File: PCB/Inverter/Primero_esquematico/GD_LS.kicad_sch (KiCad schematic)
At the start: 46 parts, among them T7 750317595, U40 LM25180QNGURQ1, U41 UCC21750QDWRQ1, U42 LP2951-5.0_VSSOP

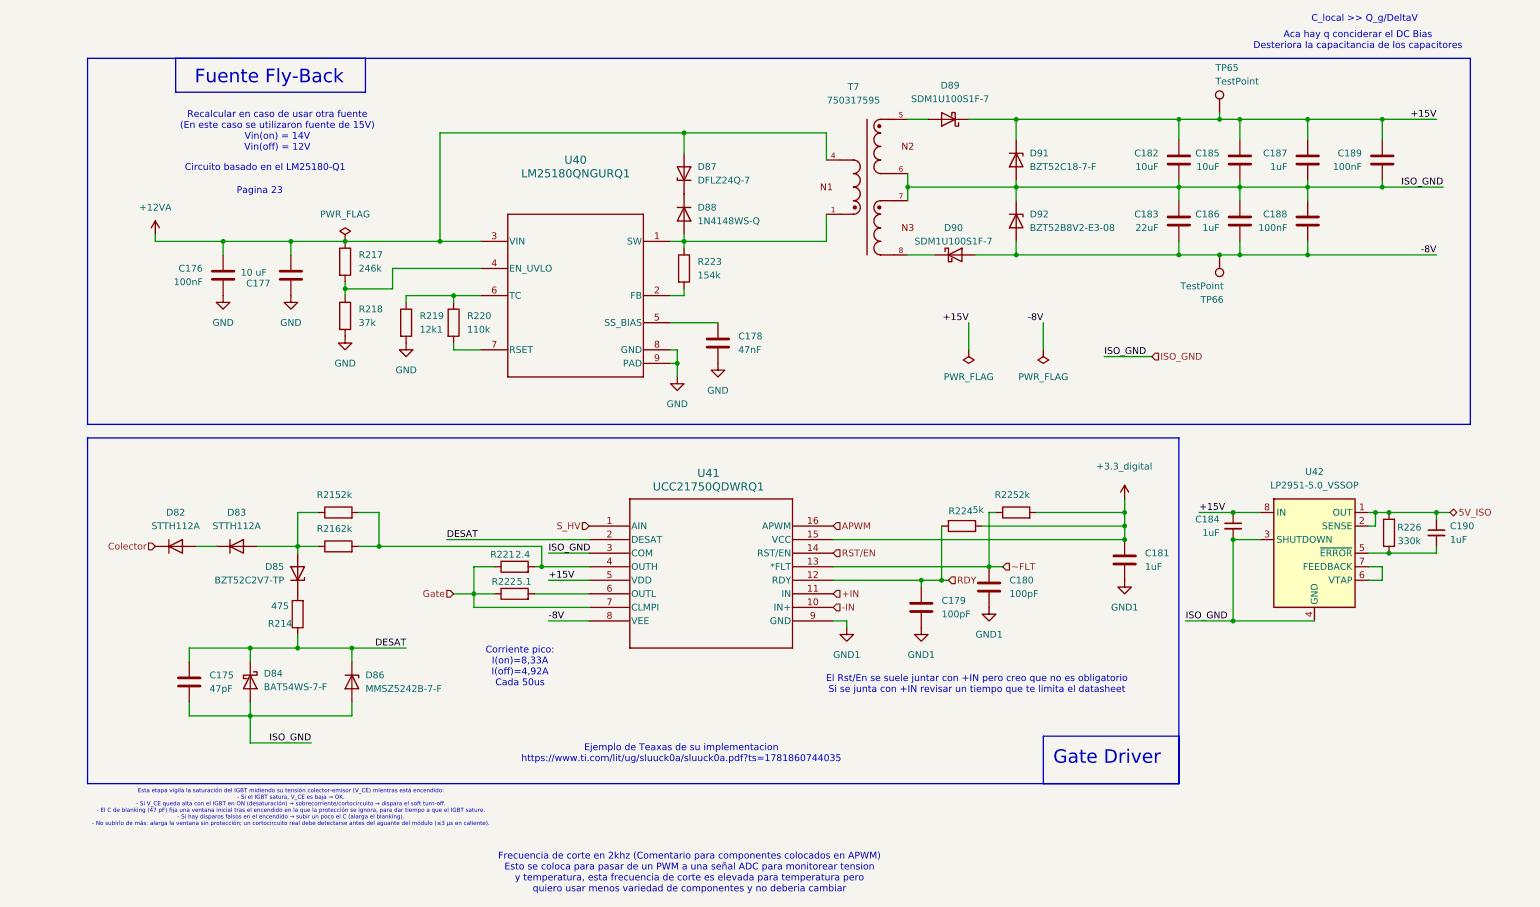
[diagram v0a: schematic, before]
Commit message: Corregi cosas de la placa
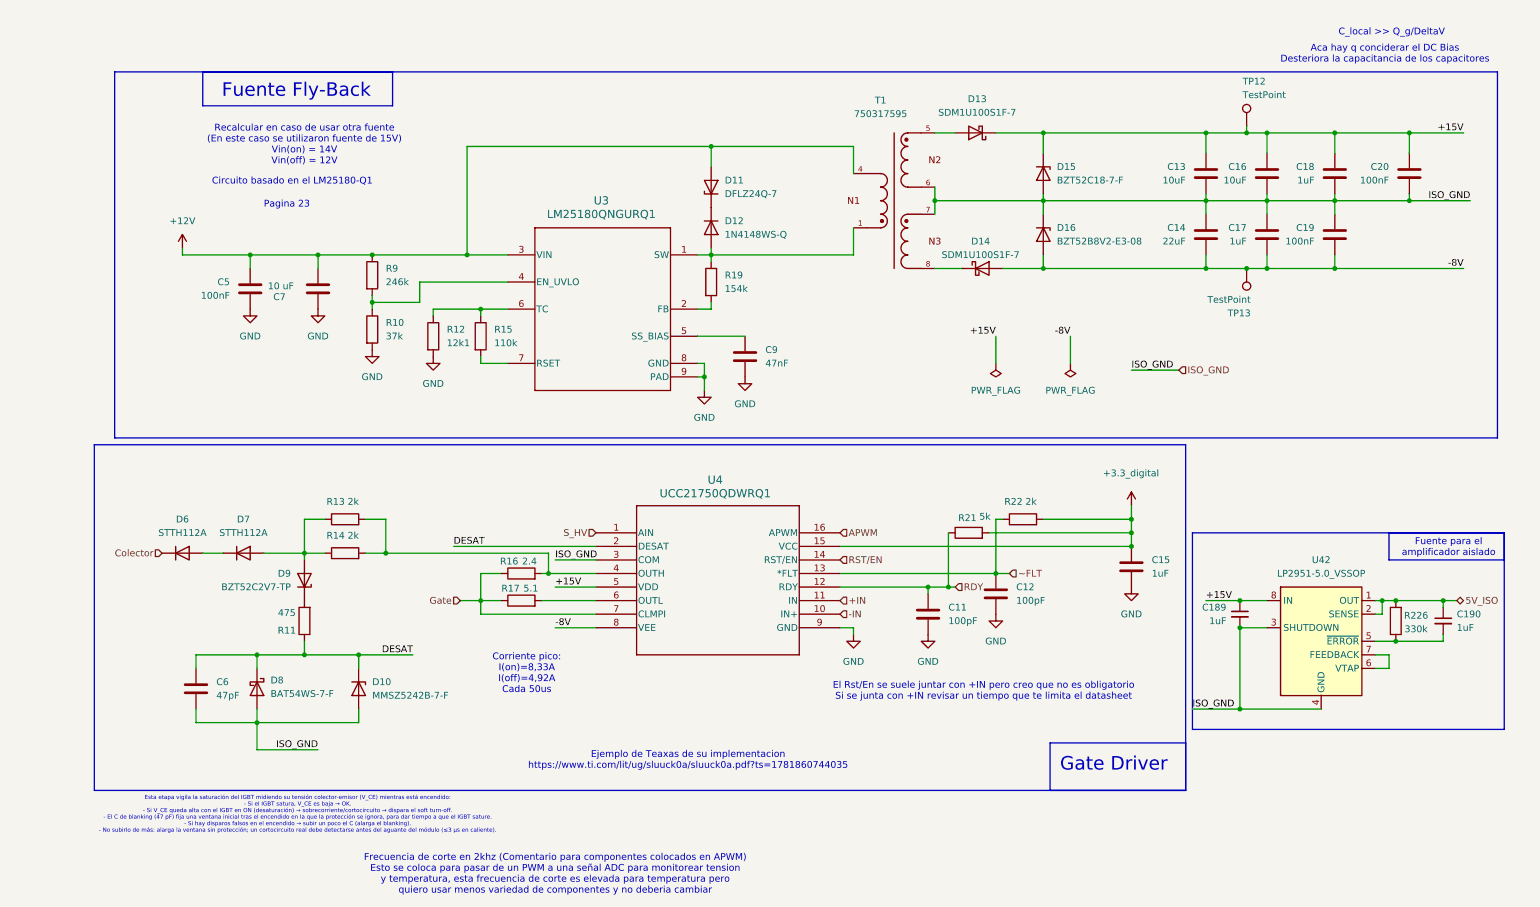
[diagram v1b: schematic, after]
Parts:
- removed C175: 47pF, Capacitor_SMD:C_0603_1608Metric_Pad1.08x0.95mm_HandSolder, symbol Device:C
- removed C176, C188, C189: 100nF, Capacitor_SMD:C_0402_1005Metric, symbol Device:C
- removed C177: 10 uF, Capacitor_SMD:C_1206_3216Metric, symbol Device:C
- removed C178: 47nF, Capacitor_SMD:C_0402_1005Metric_Pad0.74x0.62mm_HandSolder, symbol Device:C
- removed C179, C180: 100pF, Capacitor_SMD:C_0402_1005Metric, symbol Device:C
- removed C181: 1uF, Capacitor_SMD:C_0603_1608Metric, symbol Device:C
- removed C182, C185: 10uF, Capacitor_SMD:C_1210_3225Metric, symbol Device:C
- removed C183: 22uF, Capacitor_SMD:C_1210_3225Metric, symbol Device:C
- removed C184: 1uF, Capacitor_SMD:C_0603_1608Metric, symbol Device:C_Small
- removed C186, C187: 1uF, Capacitor_SMD:C_0805_2012Metric, symbol Device:C
- removed D82, D83: STTH112A, Diode_SMD:D_SOD-323F, symbol Device:D
- removed D84: BAT54WS-7-F, Diode_SMD:D_SOD-323_HandSoldering, symbol Device:D_Schottky
- removed D85: BZT52C2V7-TP, Diode_SMD:D_SOD-123, symbol Device:D_Zener
- removed D86: MMSZ5242B-7-F, Diode_SMD:D_SOD-123, symbol Device:D_Zener
- removed D87: DFLZ24Q-7, Diode_SMD:D_PowerDI-123, symbol Device:D_Zener
- removed D88: 1N4148WS-Q, Diode_SMD:D_SOD-323F, symbol Device:D
- removed D89, D90: SDM1U100S1F-7, Diode_SMD:D_SOD-123F, symbol Device:D_Schottky
- removed D91: BZT52C18-7-F, Diode_SMD:D_SOD-123, symbol Device:D_Zener
- removed D92: BZT52B8V2-E3-08, Diode_SMD:D_SOD-123, symbol Device:D_Zener
- removed R214: 475, Resistor_SMD:R_0805_2012Metric, symbol Device:R
- removed R215, R216: 2k, Resistor_SMD:R_0805_2012Metric, symbol Device:R
- removed R217: 246k, Resistor_SMD:R_0402_1005Metric, symbol Device:R
- removed R218: 37k, Resistor_SMD:R_0402_1005Metric, symbol Device:R
- removed R219: 12k1, Resistor_SMD:R_0402_1005Metric, symbol Device:R
- removed R220: 110k, Resistor_SMD:R_0402_1005Metric, symbol Device:R
- removed R221: 2.4, Resistor_SMD:R_1206_3216Metric, symbol Device:R
- removed R222: 5.1, Resistor_SMD:R_1206_3216Metric, symbol Device:R
- removed R223: 154k, Resistor_SMD:R_0402_1005Metric_Pad0.72x0.64mm_HandSolder, symbol Device:R
- removed R224: 5k, Resistor_SMD:R_0402_1005Metric, symbol Device:R
- removed R225: 2k, Resistor_SMD:R_0402_1005Metric, symbol Device:R
- removed T7: 750317595, Snapeda:WE-FLYTI_EP7_4436, symbol Snapeda:750317595
- removed TP65, TP66: TestPoint, TestPoint:TestPoint_Pad_D1.0mm, symbol Connector:TestPoint
- removed U40: LM25180QNGURQ1, Snapeda:NGU0008C, symbol Snapeda:LM25180QNGURQ1
- removed U41: UCC21750QDWRQ1, Snapeda:SOIC16_DW_TEX-L, symbol Snapeda:UCC21750QDWRQ1
- added C11, C12: 100pF, Capacitor_SMD:C_0402_1005Metric, symbol Device:C
- added C13, C16: 10uF, Capacitor_SMD:C_1210_3225Metric, symbol Device:C
- added C14: 22uF, Capacitor_SMD:C_1210_3225Metric, symbol Device:C
- added C15: 1uF, Capacitor_SMD:C_0603_1608Metric, symbol Device:C
- added C17, C18: 1uF, Capacitor_SMD:C_0805_2012Metric, symbol Device:C
- added C189: 1uF, Capacitor_SMD:C_0603_1608Metric, symbol Device:C_Small
- added C19, C20, C5: 100nF, Capacitor_SMD:C_0402_1005Metric, symbol Device:C
- added C6: 47pF, Capacitor_SMD:C_0603_1608Metric_Pad1.08x0.95mm_HandSolder, symbol Device:C
- added C7: 10 uF, Capacitor_SMD:C_1206_3216Metric, symbol Device:C
- added C9: 47nF, Capacitor_SMD:C_0402_1005Metric_Pad0.74x0.62mm_HandSolder, symbol Device:C
- added D10: MMSZ5242B-7-F, Diode_SMD:D_SOD-123, symbol Device:D_Zener
- added D11: DFLZ24Q-7, Diode_SMD:D_PowerDI-123, symbol Device:D_Zener
- added D12: 1N4148WS-Q, Diode_SMD:D_SOD-323F, symbol Device:D
- added D13, D14: SDM1U100S1F-7, Diode_SMD:D_SOD-123F, symbol Device:D_Schottky
- added D15: BZT52C18-7-F, Diode_SMD:D_SOD-123, symbol Device:D_Zener
- added D16: BZT52B8V2-E3-08, Diode_SMD:D_SOD-123, symbol Device:D_Zener
- added D6, D7: STTH112A, Diode_SMD:D_SOD-323F, symbol Device:D
- added D8: BAT54WS-7-F, Diode_SMD:D_SOD-323_HandSoldering, symbol Device:D_Schottky
- added D9: BZT52C2V7-TP, Diode_SMD:D_SOD-123, symbol Device:D_Zener
- added R10: 37k, Resistor_SMD:R_0402_1005Metric, symbol Device:R
- added R11: 475, Resistor_SMD:R_0805_2012Metric, symbol Device:R
- added R12: 12k1, Resistor_SMD:R_0402_1005Metric, symbol Device:R
- added R13, R14: 2k, Resistor_SMD:R_0805_2012Metric, symbol Device:R
- added R15: 110k, Resistor_SMD:R_0402_1005Metric, symbol Device:R
- added R16: 2.4, Resistor_SMD:R_1206_3216Metric, symbol Device:R
- added R17: 5.1, Resistor_SMD:R_1206_3216Metric, symbol Device:R
- added R19: 154k, Resistor_SMD:R_0402_1005Metric_Pad0.72x0.64mm_HandSolder, symbol Device:R
- added R21: 5k, Resistor_SMD:R_0402_1005Metric, symbol Device:R
- added R22: 2k, Resistor_SMD:R_0402_1005Metric, symbol Device:R
- added R9: 246k, Resistor_SMD:R_0402_1005Metric, symbol Device:R
- added T1: 750317595, Snapeda:WE-FLYTI_EP7_4436, symbol Snapeda:750317595
- added TP12, TP13: TestPoint, TestPoint:TestPoint_Pad_D1.0mm, symbol Connector:TestPoint
- added U3: LM25180QNGURQ1, Snapeda:NGU0008C, symbol Snapeda:LM25180QNGURQ1
- added U4: UCC21750QDWRQ1, Snapeda:SOIC16_DW_TEX-L, symbol Snapeda:UCC21750QDWRQ1
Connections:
- net +15V: now also C13.2, C16.2, C18.2, C189.1, C20.2, D13.1 (K), D15.1 (K), TP12.1, U4.5 (VDD)
- net +3.3_digital: now also C15.2, R21.2, R22.2, U4.15 (VCC)
- net +IN: now also U4.11 (IN)
- net -8V: now also C14.1, C17.1, C19.1, D14.2 (A), D16.2 (A), TP13.1, U4.8 (VEE)
- net -IN: now also U4.10 (IN+)
- net APWM: now also U4.16 (APWM)
- net Colector: now also D6.1 (K)
- net DESAT: now also C6.2, D10.1 (K), D8.1 (K), R11.1, U4.2 (DESAT)
- net GND: now also C11.1, C12.1, C15.1, C5.1, C7.2, C9.1, R10.2, R12.2, U3.8 (GND), U3.9 (PAD), U4.9 (GND)
- net Gate: now also R16.1, R17.1, U4.7 (CLMPI)
- net ISO_GND: now also C13.1, C14.2, C16.1, C17.2, C18.1, C189.2, C19.2, C20.1, C6.1, D10.2 (A), D15.2 (A), D16.1 (K), D8.2 (A), T1.6, T1.7, U4.3 (COM)
- net RDY: now also C11.2, R21.1, U4.12 (RDY)
- net RST/EN: now also U4.14 (RST/EN)
- net S_HV: now also U4.1 (AIN)
- net ~FLT: now also C12.2, R22.1, U4.13 (*FLT)
- new net: D6.2 (A), D7.1 (K)
- new net: D12.2 (A), R19.1, T1.1, U3.1 (SW)
- new net: R19.2, U3.2 (FB)
- new net: R10.1, R9.2, U3.4 (EN_UVLO)
- new net: C9.2, U3.5 (SS_BIAS)
- new net: R12.1, R15.1, U3.6 (TC)
- new net: R15.2, U3.7 (RSET)
- new net: R17.2, U4.6 (OUTL)
- new net: D7.2 (A), D9.2 (A), R13.1, R14.1
- new net: R13.2, R14.2, R16.2, U4.4 (OUTH)
- new net: D9.1 (K), R11.2
- new net: D13.2 (A), T1.5
- new net: D14.1 (K), T1.8
- new net: D11.1 (K), D12.1 (K)
- new net +12V: C5.2, C7.1, D11.2 (A), R9.1, T1.4, U3.3 (VIN)
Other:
- note added: "Fuente para el amplificador aislado"
